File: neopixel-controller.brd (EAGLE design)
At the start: 23.8 x 26.7 mm, 12 parts, among them J1 Power, U1 ATTiny85

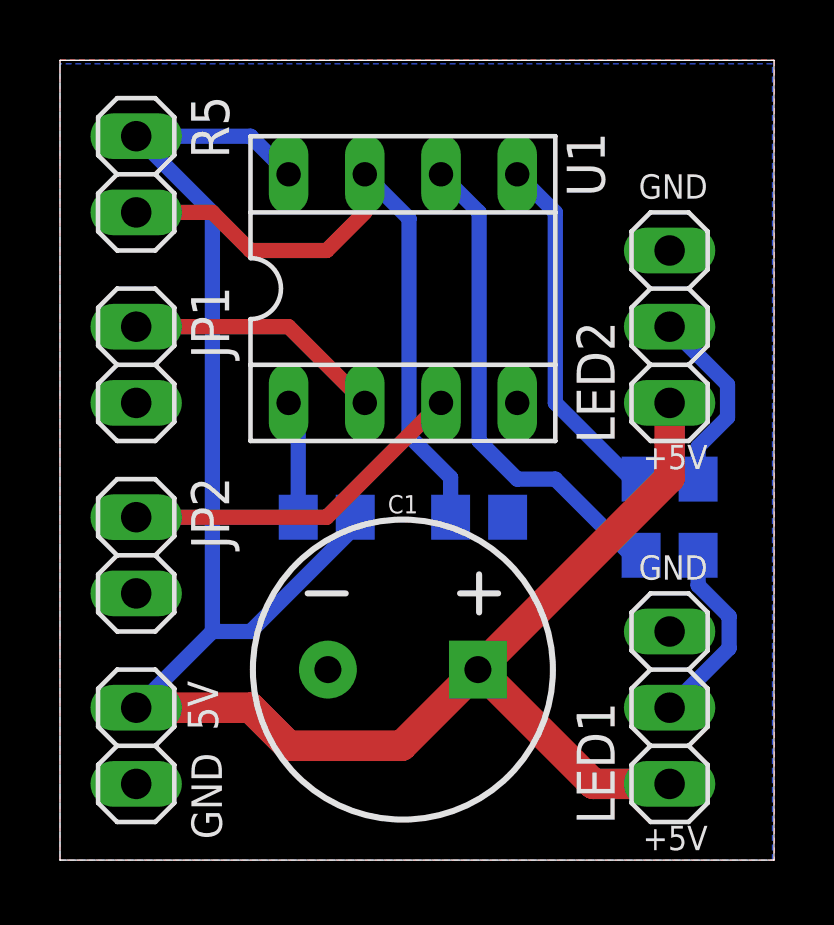
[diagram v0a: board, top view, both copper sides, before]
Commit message: Final revision
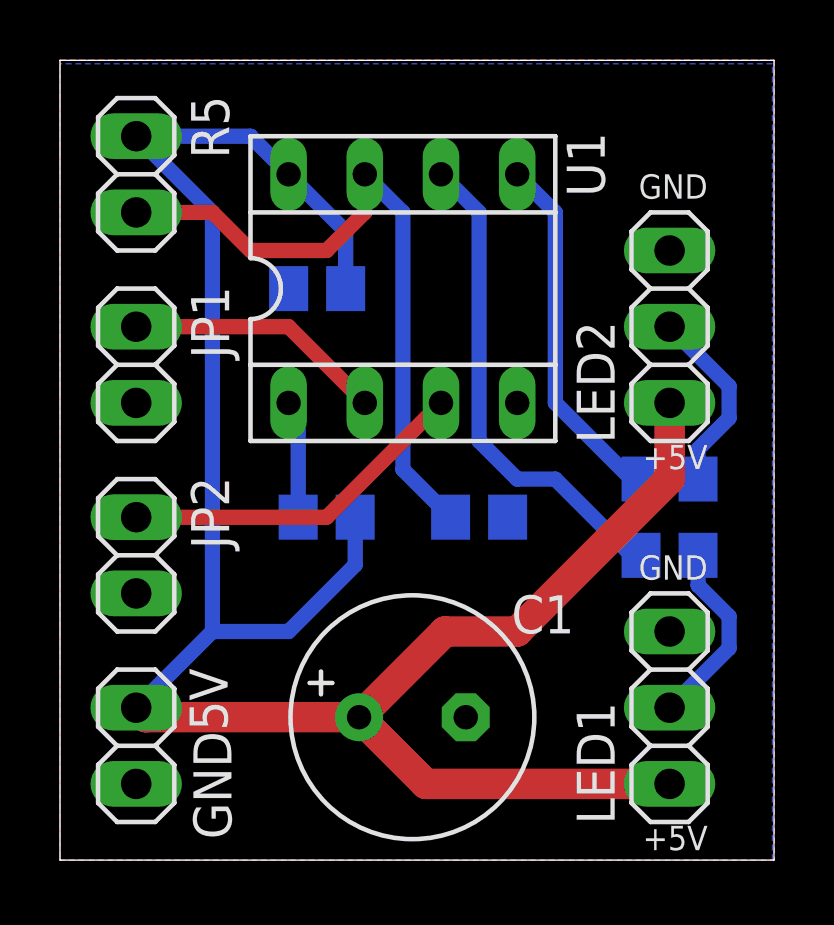
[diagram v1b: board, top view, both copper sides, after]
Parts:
- added C2: 0.1uF, resistor:C0805
- C1: value 1mF -> 1000uF; device SparkFun-Capacitors:CPOL-RADIAL-5MM-10MM -> JoshCustom:CAP-3,5-8
- moved C1 1.62 mm to (11.7, 4.76)
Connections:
- net GND: now also C1.NEGATIVE, C2.2; no longer C1.-
- net VCC: now also C1.POSITIVE, C2.1; no longer C1.+
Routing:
- net VCC: track 65.9 -> 73.6 mm
